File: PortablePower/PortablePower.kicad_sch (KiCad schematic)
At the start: 0 parts

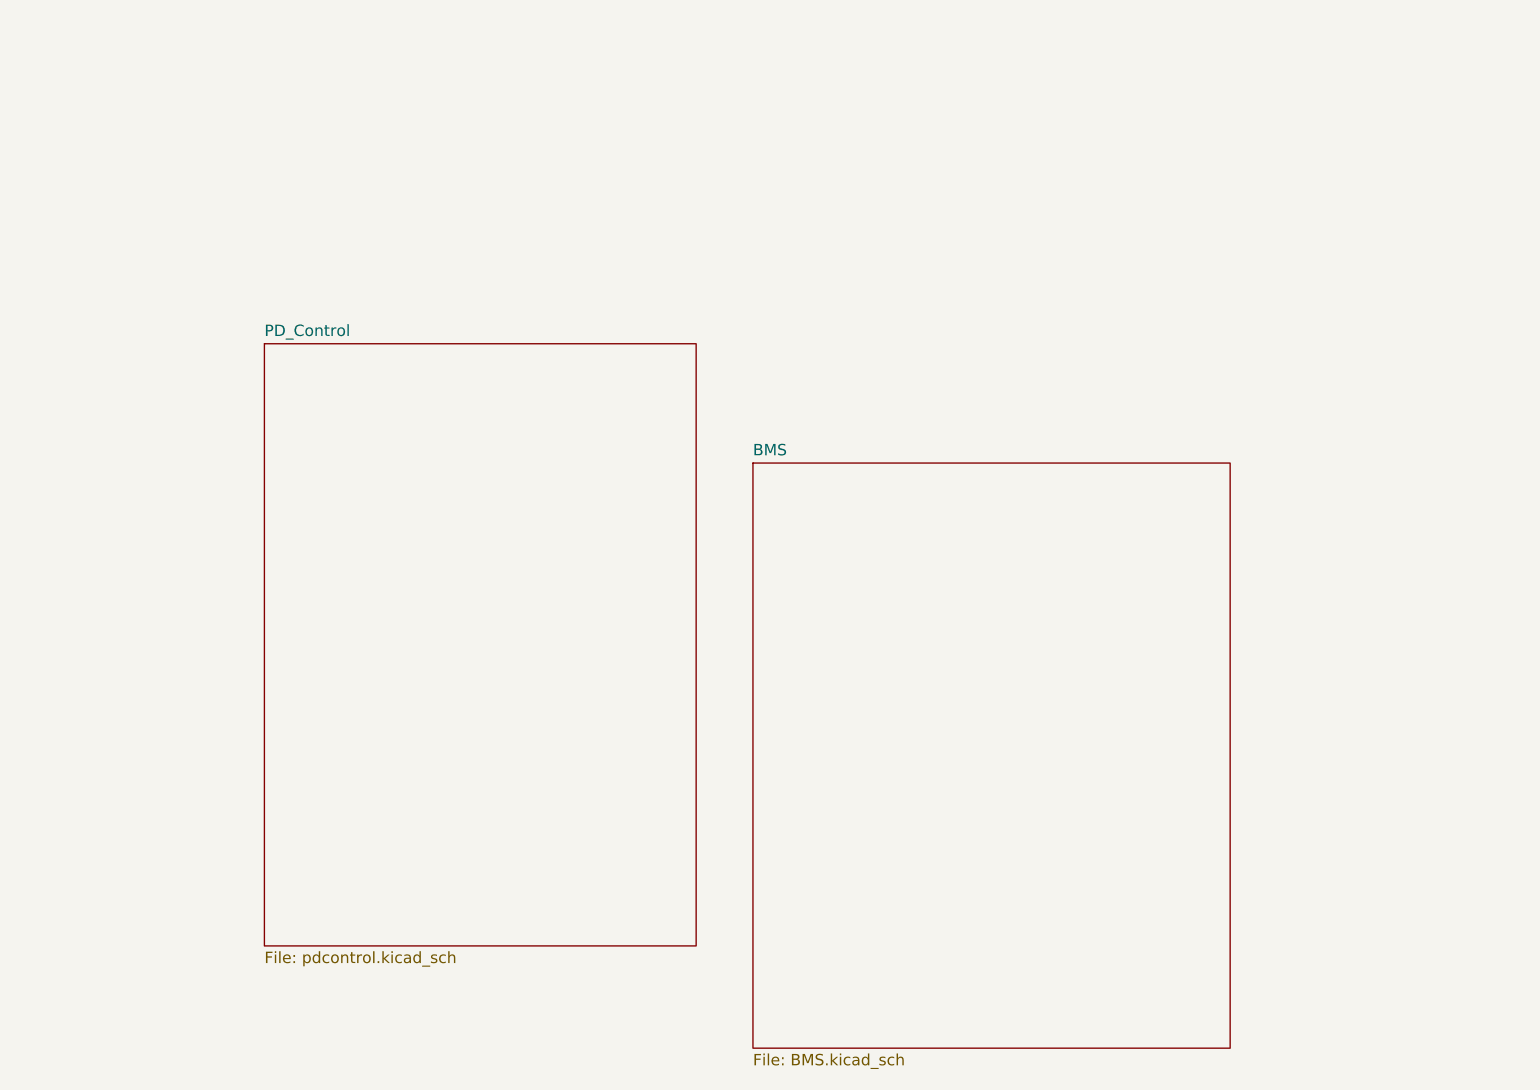
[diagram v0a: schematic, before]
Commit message: pc done
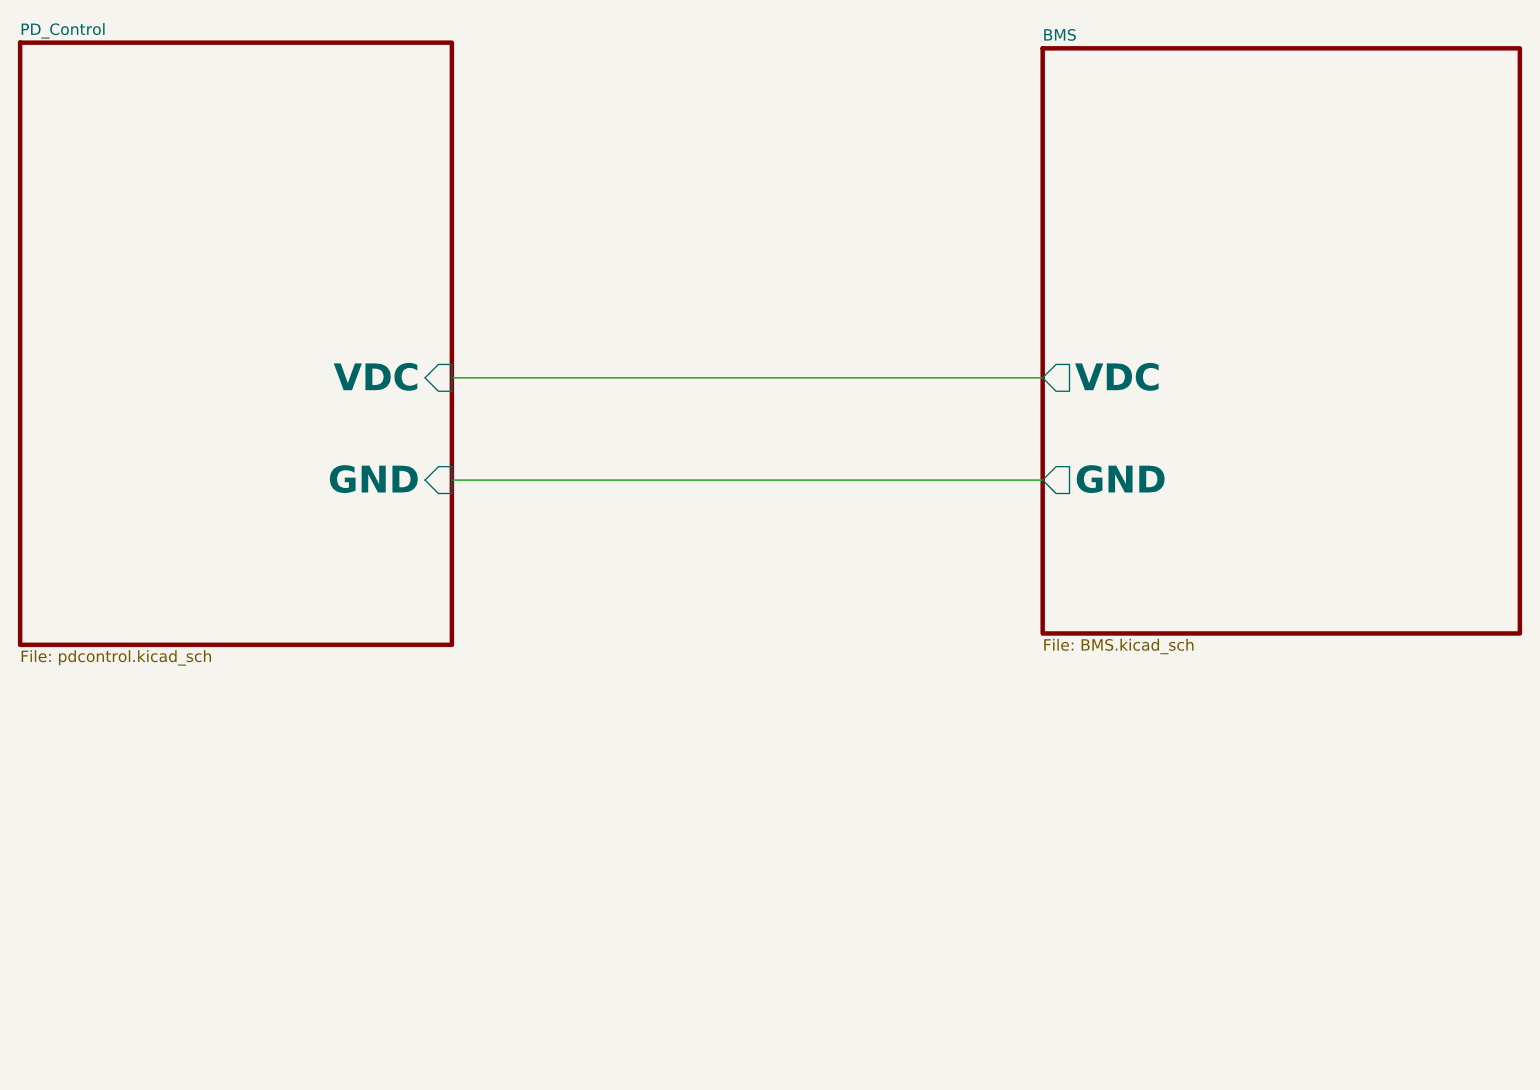
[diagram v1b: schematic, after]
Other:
- sheet BMS ports: added GND, VDC; removed none
- sheet PD_Control ports: added GND, VDC; removed none
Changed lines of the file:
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@@
 	(generator "eeschema")
 	(generator_version "9.0")
-	(paper "A4")
+	(paper "A5")
+	(wire
+		(pts
+			(xy 67.945 59.69) (xy 133.985 59.69)
+		)
+		(stroke
+			(width 1)
+			(type default)
+			(color 255 0 0 1)
+		)
+	)
+	(wire
+		(pts
+			(xy 67.945 71.12) (xy 133.985 71.12)
+		)
+		(stroke
+			(width 1)
+			(type default)
+			(color 0 0 0 1)
+		)
+	)
 	(sheet
-		(at 46.99 55.88)
+		(at 19.685 22.225)
 		(size 48.26 67.31)
 		(exclude_from_sim no)
@@
 		(fields_autoplaced yes)
 		(stroke
-			(width 0.1524)
+			(width 0.5)
 			(type solid)
+			(color 0 0 0 1)
 		)
 		(fill
-			(color 0 0 0 0.0000)
+			(color 0 255 0 1.0000)
 		)
 		(property "Sheetname" "PD_Control"
-			(at 46.99 55.1684 0)
+			(at 19.685 21.5134 0)
 			(effects
 				(font
@@
 		)
 		(property "Sheetfile" "pdcontrol.kicad_sch"
-			(at 46.99 123.7746 0)
+			(at 19.685 90.1196 0)
 			(effects
 				(font
@@
 				)
 				(justify left top)
+			)
+		)
+		(pin "GND" input
+			(at 67.945 71.12 0)
+			(effects
+				(font
+					(size 3 3)
+					(thickness 0.6)
+					(bold yes)
+				)
+				(justify right)
+			)
+		)
+		(pin "VDC" input
+			(at 67.945 59.69 0)
+			(effects
+				(font
+					(size 3 3)
+					(thickness 0.6)
+					(bold yes)
+				)
+				(justify right)
 			)
 		)
@@
 	)
 	(sheet
-		(at 101.6 69.215)
+		(at 133.985 22.86)
 		(size 53.34 65.405)
 		(exclude_from_sim no)
@@
 		(fields_autoplaced yes)
 		(stroke
-			(width 0.1524)
+			(width 0.5)
 			(type solid)
+			(color 0 0 0 1)
 		)
 		(fill
-			(color 0 0 0 0.0000)
+			(color 255 153 0 1.0000)
 		)
 		(property "Sheetname" "BMS"
-			(at 101.6 68.5034 0)
+			(at 133.985 22.1484 0)
 			(effects
 				(font
@@
 		)
 		(property "Sheetfile" "BMS.kicad_sch"
-			(at 101.6 135.2046 0)
+			(at 133.985 88.8496 0)
 			(effects
 				(font
@@
 			)
 		)
+		(pin "GND" output
+			(at 133.985 71.12 180)
+			(effects
+				(font
+					(size 3 3)
+					(thickness 0.6)
+					(bold yes)
+				)
+				(justify left)
+			)
+		)
+		(pin "VDC" output
+			(at 133.985 59.69 180)
+			(effects
+				(font
+					(size 3 3)
+					(thickness 0.6)
+					(bold yes)
+				)
+				(justify left)
+			)
+		)
